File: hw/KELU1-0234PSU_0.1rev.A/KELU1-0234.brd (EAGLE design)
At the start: 50 x 85 mm, 78 parts, among them IC1 UC3844, P1 B3B-EH-A, P2 B3B-EH-A, Q2 IRF740TO220BVH, T1 E25137

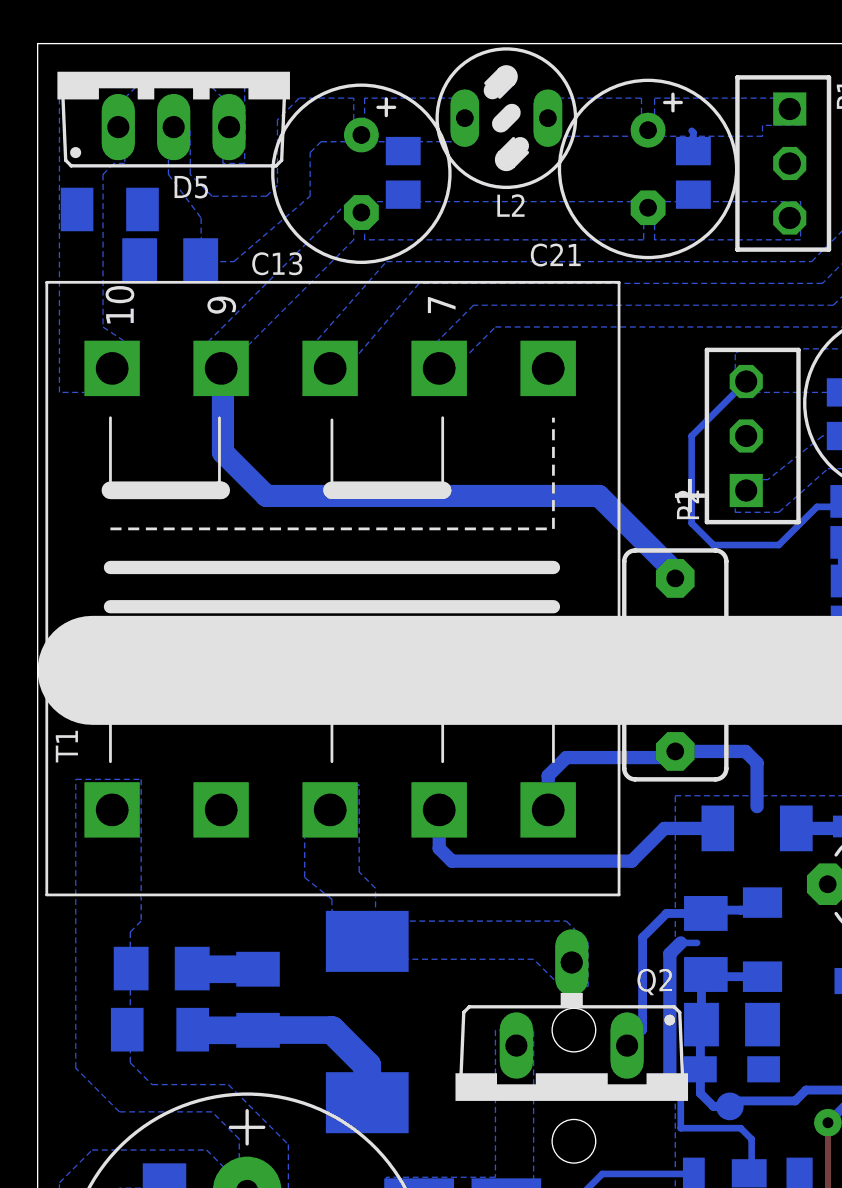
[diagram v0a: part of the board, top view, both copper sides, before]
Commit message: Update
Update circuit
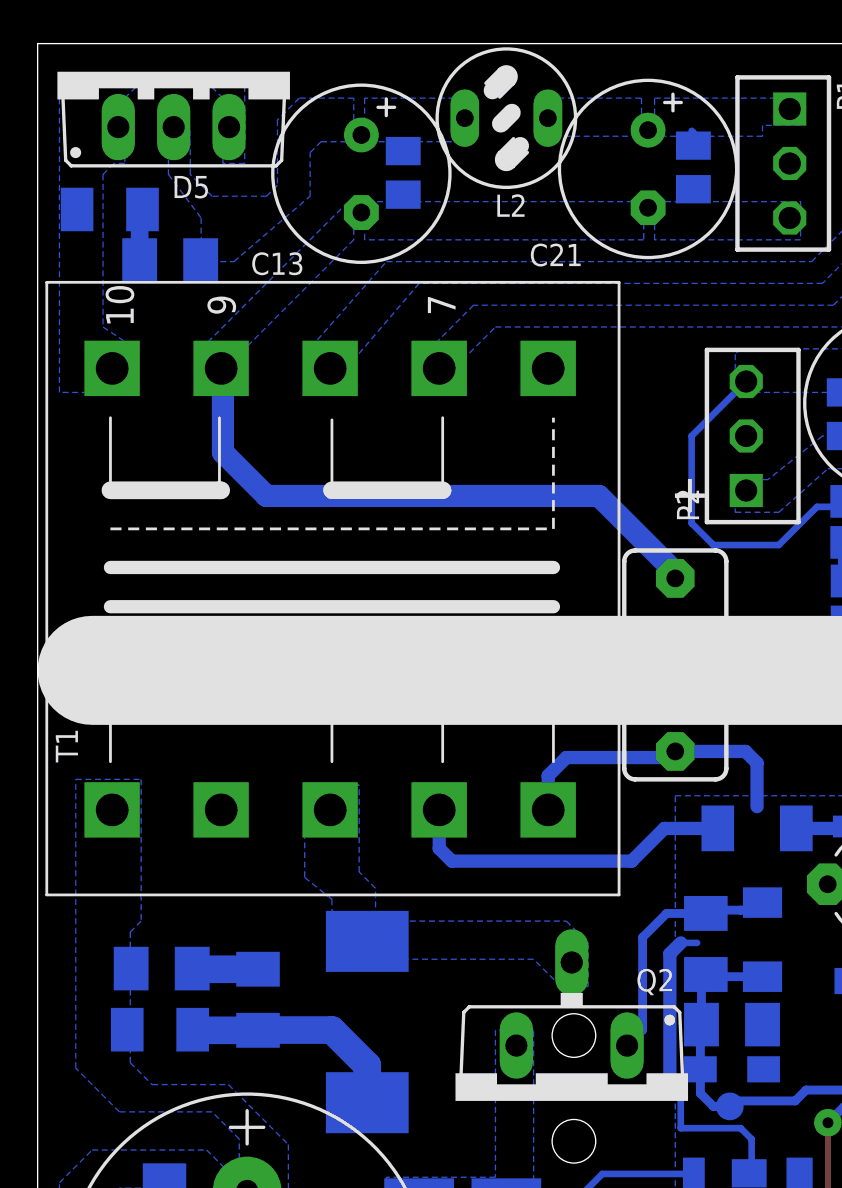
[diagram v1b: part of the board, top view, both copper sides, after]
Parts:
- moved C15 0.25 mm to (30.1, 79.3)
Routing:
- net N$33: track 0.00 -> 2.45 mm
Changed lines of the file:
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@@
 <hole x="6.3" y="18.2" drill="2"/>
 <hole x="13.6" y="18.2" drill="2"/>
-<hole x="24.6" y="39.75" drill="2"/>
+<hole x="24.6" y="39.5" drill="2"/>
 <hole x="24.6" y="34.65" drill="2"/>
 <hole x="24.6" y="27.15" drill="2"/>
@@
 <attribute name="VALUE" x="18.67" y="80.07" size="1.016" layer="28" rot="MR270"/>
 </element>
-<element name="C15" library="resistor" package="C0805K" value="0.1u" x="30.08" y="79.07" smashed="yes" rot="MR270">
-<attribute name="NAME" x="32.455" y="80.57" size="1.016" layer="26" font="vector" ratio="15" rot="MR270"/>
-<attribute name="VALUE" x="31.98" y="80.07" size="1.016" layer="28" rot="MR270"/>
+<element name="C15" library="resistor" package="C0805K" value="0.1u" x="30.08" y="79.32" smashed="yes" rot="MR270">
+<attribute name="NAME" x="32.455" y="80.82" size="1.016" layer="26" font="vector" ratio="15" rot="MR270"/>
+<attribute name="VALUE" x="31.98" y="80.32" size="1.016" layer="28" rot="MR270"/>
 </element>
 <element name="L2" library="inductors" package="82114R" value="4u" x="21.5" y="81.58" smashed="yes" rot="R90">
@@
 </polygon>
 <contactref element="P1" pad="1"/>
-<wire x1="30.08" y1="80.07" x2="30.08" y2="80.92" width="0.3048" layer="16"/>
+<wire x1="30.08" y1="80.32" x2="30.08" y2="80.92" width="0.3048" layer="16"/>
 <wire x1="30.08" y1="80.92" x2="30" y2="81" width="0.3048" layer="16"/>
 </signal>
@@
 <contactref element="C20" pad="2"/>
 <contactref element="R21" pad="1"/>
-<wire x1="4.68" y1="75.07" x2="4.81" y2="77.39" width="0" layer="19" extent="16-16"/>
+<wire x1="4.81" y1="77.39" x2="4.68" y2="77.39" width="0.8128" layer="16"/>
+<wire x1="4.68" y1="77.39" x2="4.68" y2="75.07" width="0.8128" layer="16"/>
 </signal>
 <signal name="GND1">
